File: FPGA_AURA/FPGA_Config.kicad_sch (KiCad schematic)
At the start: 31 parts, among them U1 XC7A35T-2FTG256C, U2 W25Q256JVEIQ, U3 FT2232HQ, U5 USBLC6-2SC6, U6 93LC56BT-I_SN, Y1 12MHz

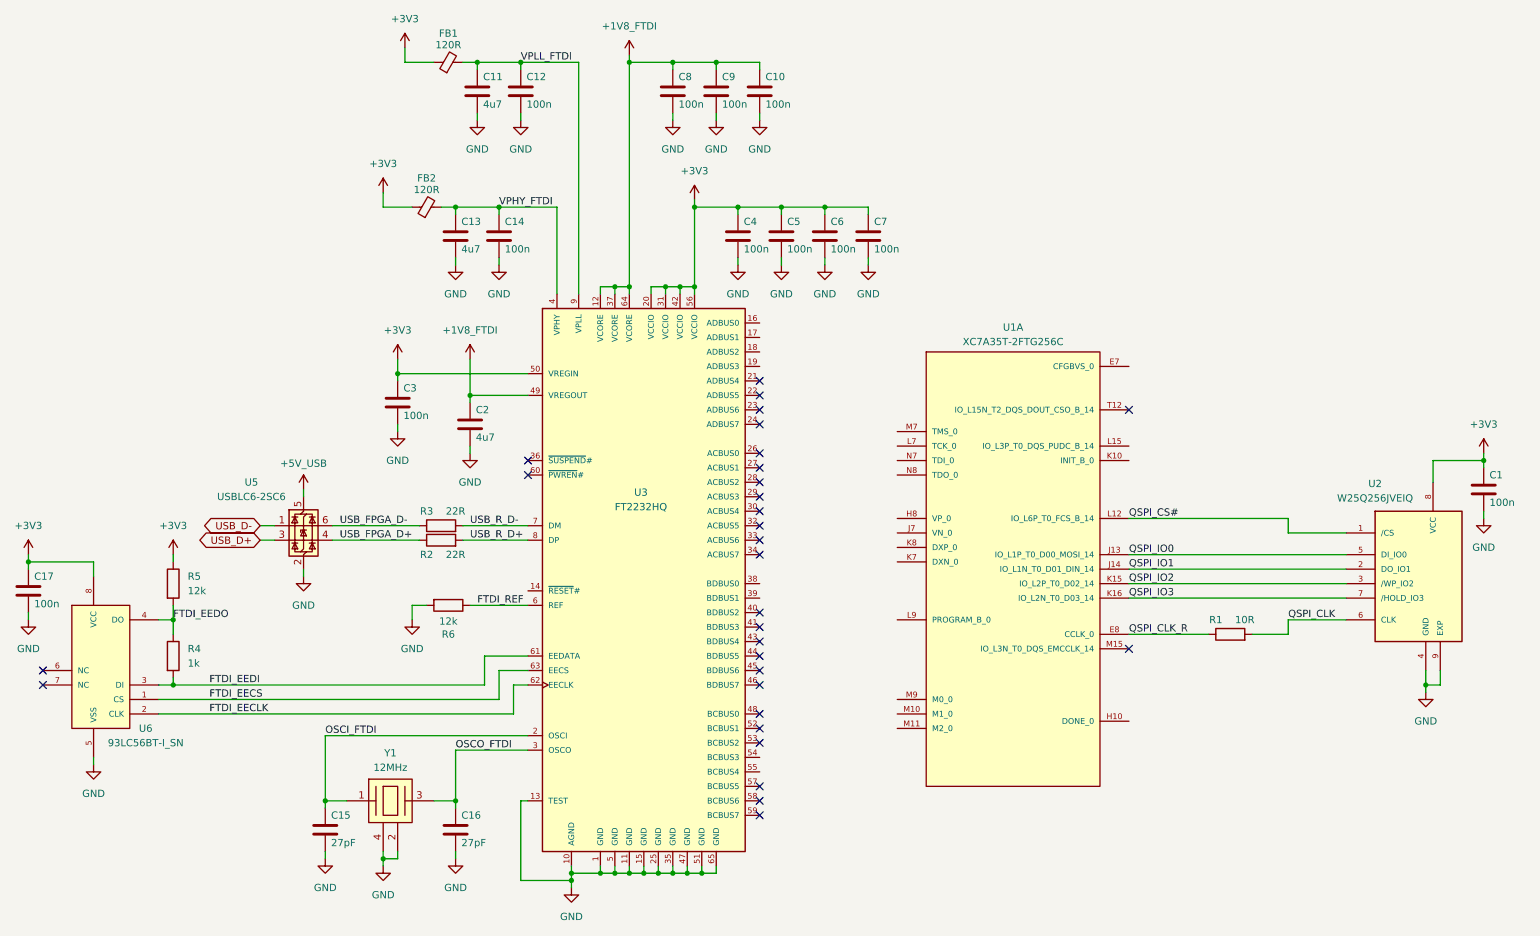
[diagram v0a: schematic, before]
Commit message: Continuing the FTDI
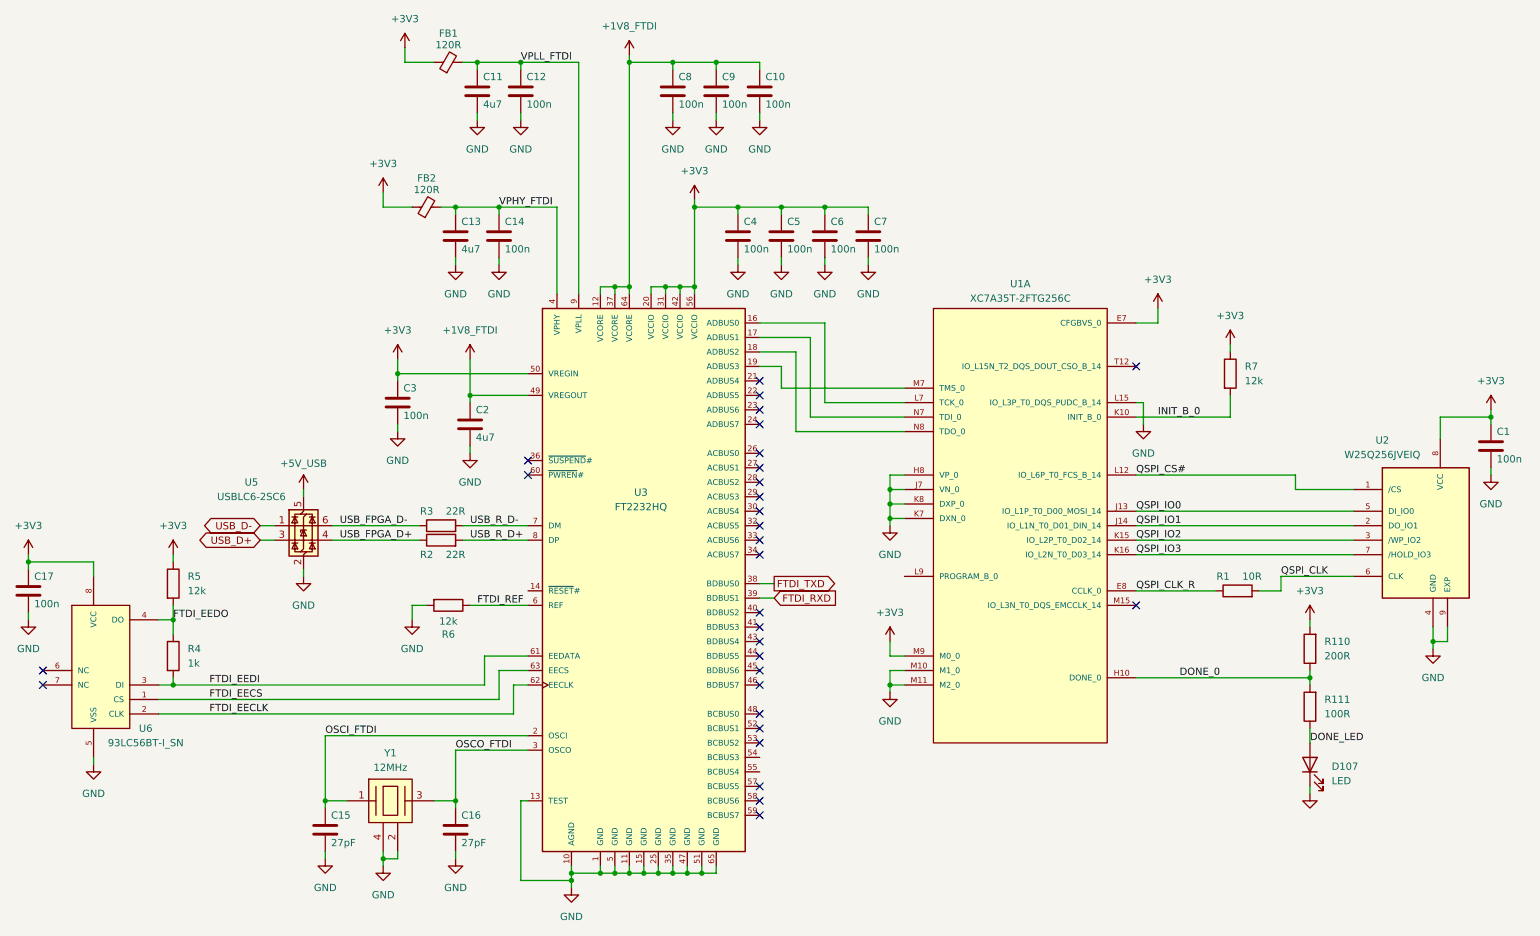
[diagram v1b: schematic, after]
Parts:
- added D107: LED, LED_SMD:LED_0603_1608Metric, symbol Device:LED
- added R110: 200R, Resistor_SMD:R_0402_1005Metric, symbol Device:R
- added R111: 100R, Resistor_SMD:R_0402_1005Metric, symbol Device:R
- added R7: 12k, Resistor_SMD:R_0402_1005Metric, symbol Device:R
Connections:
- net +3V3: now also U1.E7 (CFGBVS_0), U1.M9 (M0_0), R110.2, R7.1
- net GND: now also U1.H8 (VP_0), U1.J7 (VN_0), U1.K7 (DXN_0), U1.K8 (DXP_0), U1.L15 (IO_L3P_T0_DQS_PUDC_B_14), U1.M10 (M1_0), U1.M11 (M2_0), D107.1 (K)
- net at U3.16 (ADBUS0): now also U1.L7 (TCK_0)
- net at U3.17 (ADBUS1): now also U1.N7 (TDI_0)
- net at U3.18 (ADBUS2): now also U1.N8 (TDO_0)
- net at U3.19 (ADBUS3): now also U1.M7 (TMS_0)
- net FTDI_TXD: now reaches U3.38 (BDBUS0)
- net FTDI_RXD: now reaches U3.39 (BDBUS1)
- net DONE_0: now reaches U1.H10 (DONE_0)
- net DONE_0: now also R110.1, R111.2
- net INIT_B_0: now reaches U1.K10 (INIT_B_0)
- net INIT_B_0: now also R7.2
- new net DONE_LED: D107.2 (A), R111.1
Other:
- moved on the sheet: C1, R1, U1A, U2
